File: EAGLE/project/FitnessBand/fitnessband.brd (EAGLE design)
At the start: 40 x 30.1 mm, 59 parts, among them J5 TC2030-JLINK-NL, U17 NRF51822QF, X3 EPSON-FA-128, X4 ABS05-32.768KHZ-T, X5 USB-MICROB

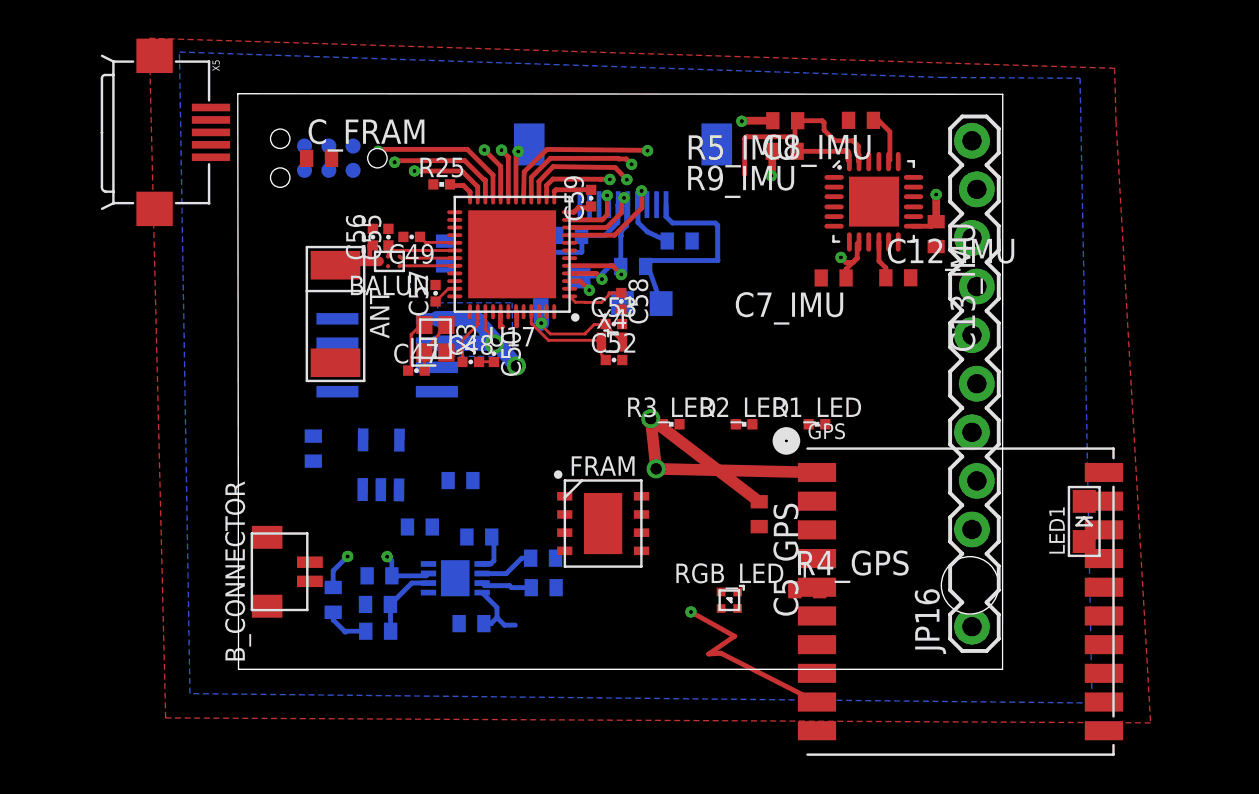
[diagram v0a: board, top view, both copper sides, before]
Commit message: asdf
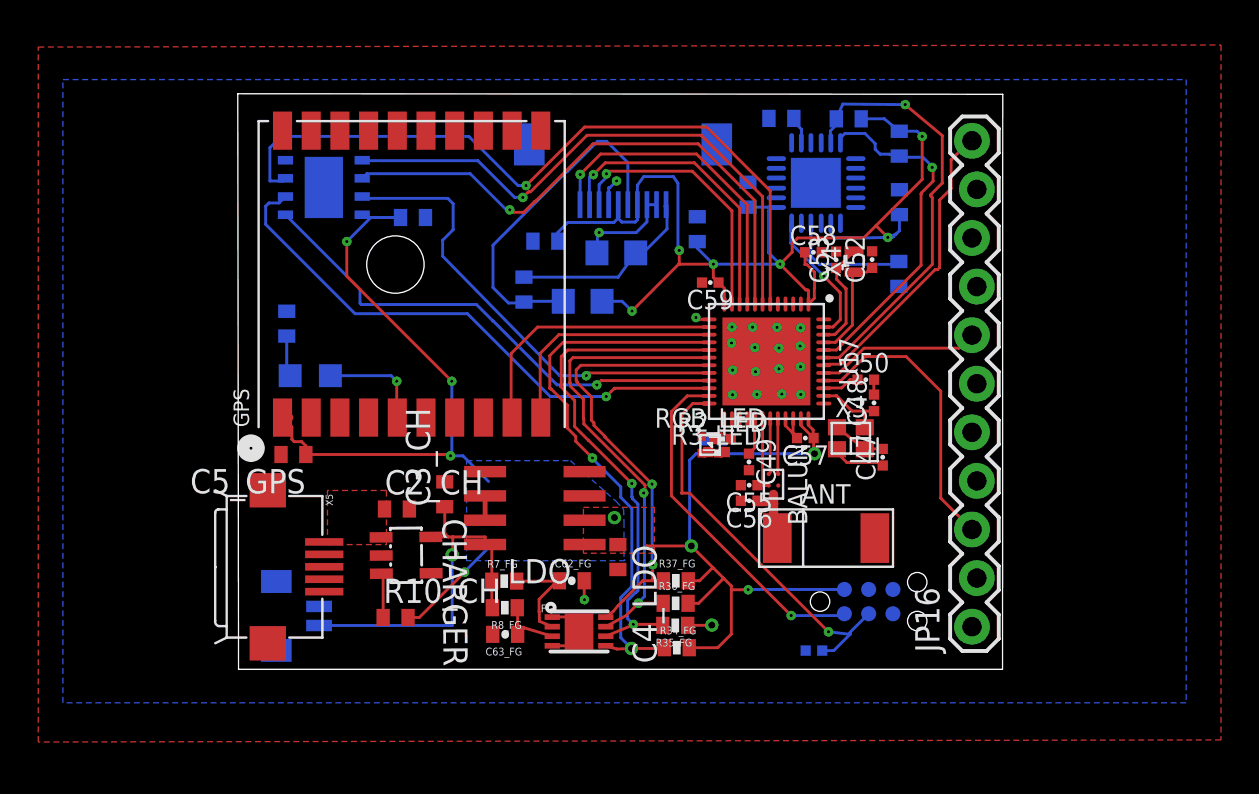
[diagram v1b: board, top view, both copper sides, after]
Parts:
- removed B_CONNECTOR: SH_MALE_2/1MM, headers:SH-1X2/1MM
- added LIPO: SH_MALE_2/1MM, headers:SH-1X2/1MM
- moved LED1 41.2 mm to (3.75, 15.3), flipped to the bottom, turned to 270 degrees
- moved J5 36.5 mm to (32.9, 3.54), turned to 180 degrees
- moved GPS 33.4 mm to (9.05, 20.7), turned to 90 degrees
- moved R25 31.2 mm to (30.1, 0.98), flipped to the bottom, turned to 180 degrees
- moved R4_GPS 30.6 mm to (2.52, 18.1), flipped to the bottom, turned to 270 degrees
- moved ANT 28.2 mm to (30.7, 6.86), turned to 0 degrees
- moved C47 24.8 mm to (33.7, 11.1), turned to 90 degrees
- moved C5_GPS 24.5 mm to (2.87, 11.2), turned to 180 degrees
- moved C56 24.0 mm to (26.7, 8.81), turned to 180 degrees
- moved X5 23.5 mm to (1.38, 5.36)
- moved BALUN 23.2 mm to (28.0, 9.68), turned to 270 degrees
- moved C55 22.9 mm to (26.7, 9.63), turned to 180 degrees
- moved FRAM 22.8 mm to (4.46, 25.2), flipped to the bottom, turned to 90 degrees
- moved X3 22.3 mm to (32.0, 12.1), turned to 0 degrees
- moved C49 21.2 mm to (26.7, 10.8), turned to 270 degrees
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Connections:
- net !FRAM_WP: now also U17.6; no longer U17.22
- net ALT_FG: now also U17.16; no longer U17.18
- net BATTERY: now also LIPO.2; no longer B_CONNECTOR.2
- net BUTTON1: now also U17.42; no longer U17.40
- net BUTTON3: now also U17.40; no longer U17.42
- net GND: now also LIPO.1; no longer B_CONNECTOR.1
- net QST_FG: now also U17.17; no longer U17.19
- net SCL_FG: now also U17.18; no longer U17.17
- net SDA_FG: now also U17.19; no longer U17.16
- net SPI_MISO_FRAM: now also U17.22; no longer U17.48
- net SPI_MOSI_FRAM: now also U17.7; no longer U17.3
- net SPI_SCK_FRAM: now also U17.8; no longer U17.4
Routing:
- net 3.3V: track 67.8 -> 134.6 mm, vias 9 -> 14
- net !FRAM_WP: track 9.06 -> 38.6 mm
- net SPI_MISO_FRAM: track 0.00 -> 29.3 mm, vias 0 -> 1
- net SPI_MOSI_FRAM: track 1.25 -> 30.0 mm
- net SPI_SCK_FRAM: track 1.92 -> 29.6 mm
- net ALT_FG: track 4.85 -> 29.3 mm, vias 1 -> 2
- net !FRAM_HOLD: track 2.83 -> 24.5 mm
- net QST_FG: track 5.76 -> 27.2 mm, vias 1 -> 2
- net SWDCLK: track 1.47 -> 21.1 mm, vias 0 -> 1
- net BATTERY: track 2.38 -> 20.2 mm, vias 0 -> 1
- net !FRAM_CS: track 10.7 -> 26.4 mm
- net BUTTON1: track 0.00 -> 15.6 mm
- net BUTTON3: track 0.00 -> 15.3 mm
- net SDA_IMU: track 3.26 -> 18.4 mm, vias 0 -> 1
- net SCL_FG: track 11.2 -> 25.3 mm, vias 1 -> 2
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- added copper zone on layer 1, net 3.3V
- added copper zone on layer 16, net 3.3V
- added copper zone on layer 1, net USB_PORT
- removed copper zone on layer 15, net 3.3V
- removed copper zone on layer 16, net N$6
